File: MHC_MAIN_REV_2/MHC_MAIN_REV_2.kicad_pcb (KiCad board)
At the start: 4 copper layers, 61 x 37 mm, 42 parts, among them J1 USB_B_Micro, J2 Conn_ARM_JTAG_SWD_10, J3 BATT, J4 OLED, SW1 RESET, SW2 BOOT, SW3 RotaryEncoder_Switch, SW4 SW_SPDT, SW5 Button_0, U1 MDBT50Q-P1MV2, U2 MCP73831-2-OT, U3 CAT24C256, U4 JP19-012, U5 AP2112K-3.3, U6 MXC6655XA, Y1 32.768kHz

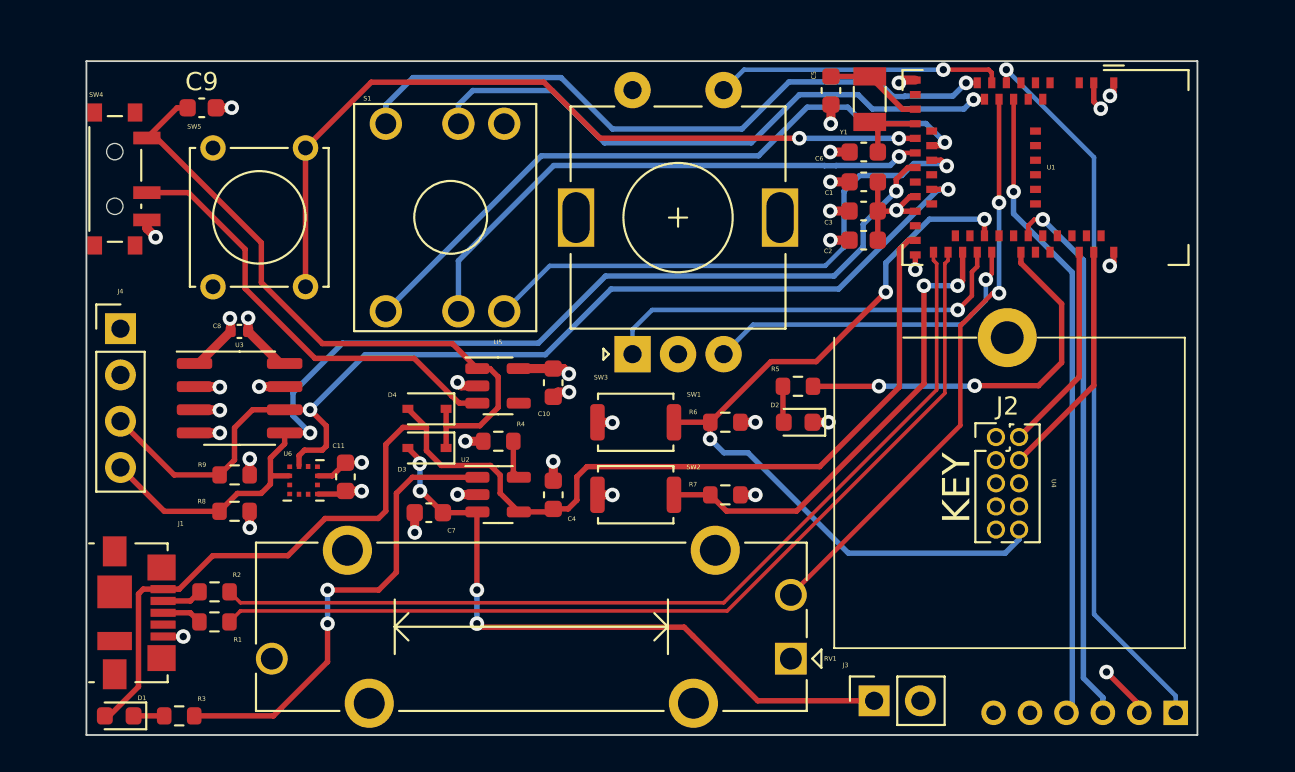
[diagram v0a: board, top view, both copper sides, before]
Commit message: Updating MHC files
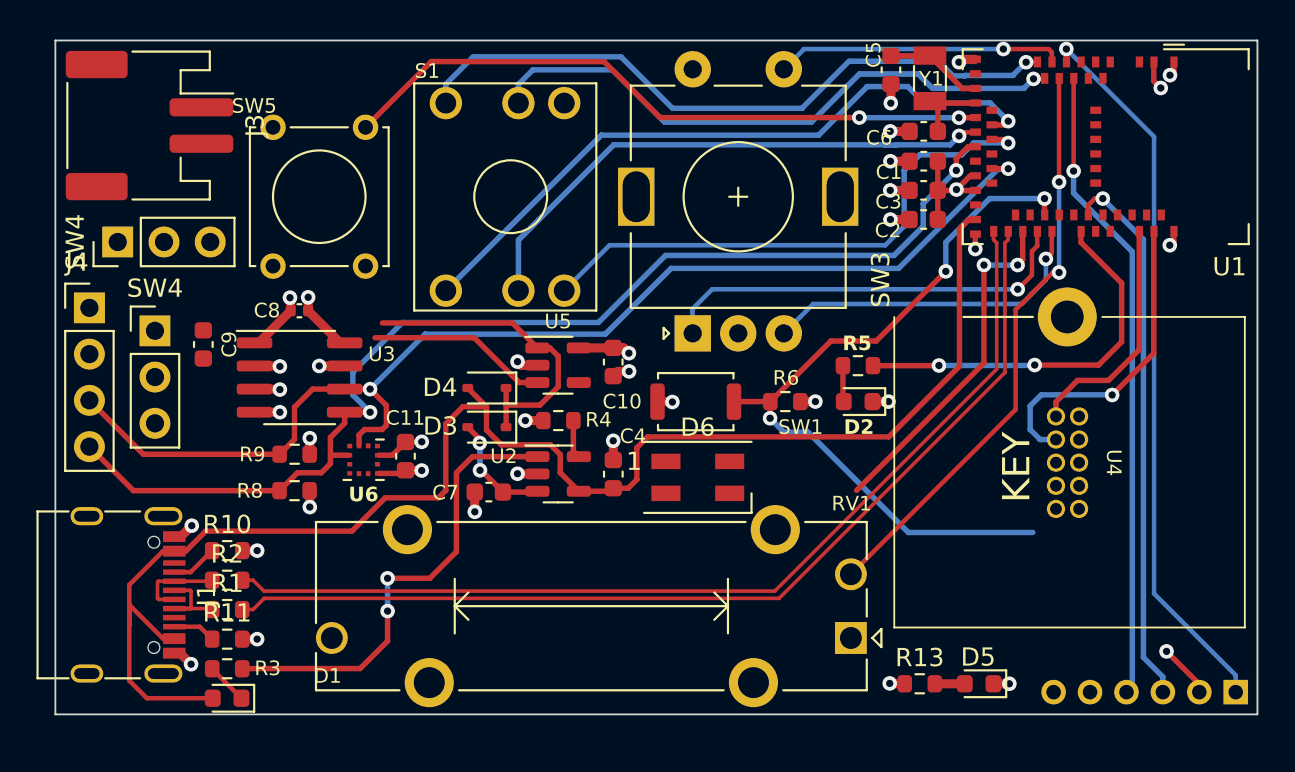
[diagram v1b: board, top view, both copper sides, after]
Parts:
- removed R7: 10k, Resistor_SMD:R_0603_1608Metric
- removed SW2: BOOT, Button_Switch_SMD:SW_Push_SPST_NO_Alps_SKRK
- removed the SW4 at (19.9, 27.7)
- added D5: RED, LED_SMD:LED_0603_1608Metric, F.Cu at (67.0, 55.5)
- added D6: SK6812MINI, LED_SMD:LED_SK6812MINI_PLCC4_3.5x3.5mm_P1.75mm, F.Cu at (51.5, 44.1)
- added R10: 5k1, Resistor_SMD:R_0603_1608Metric, F.Cu at (25.7, 48.1)
- added R11: 5k1, Resistor_SMD:R_0603_1608Metric, F.Cu at (25.7, 53.0)
- added R13: 1k, Resistor_SMD:R_0603_1608Metric, F.Cu at (63.7, 55.5)
- added SW4: SW_SPDT, Connector_PinHeader_2.54mm:PinHeader_1x03_P2.54mm_Vertical, F.Cu at (21.7, 36.1)
- added SW4: SW_SPDT, Connector_PinHeader_2.54mm:PinHeader_1x03_P2.54mm_Vertical, F.Cu at (19.7, 31.2)
- J1: value USB_B_Micro -> USB_C_Receptacle_USB2.0; footprint Connector_USB:USB_Micro-B_Molex_47346-0001 -> Connector_USB:USB_C_Receptacle_G-Switch_GT-USB-7010ASV
- J2: moved to B.Cu
- J3: footprint Connector_PinSocket_2.54mm:PinSocket_1x02_P2.54mm_Vertical -> Connector_JST:JST_PH_S2B-PH-SM4-TB_1x02-1MP_P2.00mm_Horizontal
- moved J3 50.8 mm to (21.4, 24.8), turned to -90 degrees
- moved C9 13.0 mm to (24.4, 36.8), turned to -90 degrees
- moved D1 6.00 mm to (25.7, 56.3)
- moved J2 4.70 mm to (72.5, 40.8), turned to 180 degrees
- moved R3 3.69 mm to (25.7, 54.6)
- moved SW3 3.50 mm to (51.3, 36.2)
- moved U1 3.50 mm to (73.9, 26.0)
- moved Y1 3.50 mm to (64.3, 22.2)
- moved U4 3.49 mm to (72.5, 43.3)
- moved U6 3.49 mm to (33.2, 43.2)
- moved C11 3.49 mm to (35.5, 43.0)
- moved C2 3.49 mm to (64.0, 30.0)
- moved C3 3.49 mm to (64.0, 28.4)
- moved C4 3.49 mm to (46.9, 43.9)
- moved C5 3.49 mm to (62.2, 21.8)
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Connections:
- R1 pad 1: D+ -> Net-(J1-D+-PadA6)
- R1 pad 2: Net-(J1-Pad3) -> D+
- R2 pad 1: D- -> Net-(J1-D--PadA7)
- R2 pad 2: Net-(J1-Pad2) -> D-
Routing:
- net +BATT: track 36.2 -> 6.34 mm, vias 4 -> 2
- net Net-(D3-K): track 36.0 -> 17.5 mm
- net Net-(SW4-B): track 24.2 -> 9.93 mm
- net VBUS: track 72.2 -> 83.6 mm
- net P0.04/AIN2: track 43.9 -> 36.3 mm
- net P0.13: track 26.2 -> 19.1 mm
- net Net-(J1-D--PadA7): track 0.00 -> 5.15 mm
- net SCL: track 59.7 -> 64.8 mm
- net SDA: track 58.4 -> 63.4 mm
- net Net-(J1-D+-PadA6): track 0.00 -> 4.91 mm
- net SWCLK: track 13.1 -> 17.6 mm, vias 0 -> 1
- net RESET: track 44.9 -> 41.5 mm
- net D-: track 51.5 -> 54.3 mm
- net D+: track 52.3 -> 55.1 mm
- net Net-(J1-CC1): track 0.00 -> 2.57 mm
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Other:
- board size 61 x 37 mm -> 66 x 37 mm
